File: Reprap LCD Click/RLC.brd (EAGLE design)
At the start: 100 x 80 mm, 10 parts, among them IC1 PCF8574T, Q1 BC548B, SW1 EC12E_SW, X1 HD44780LCD-1602

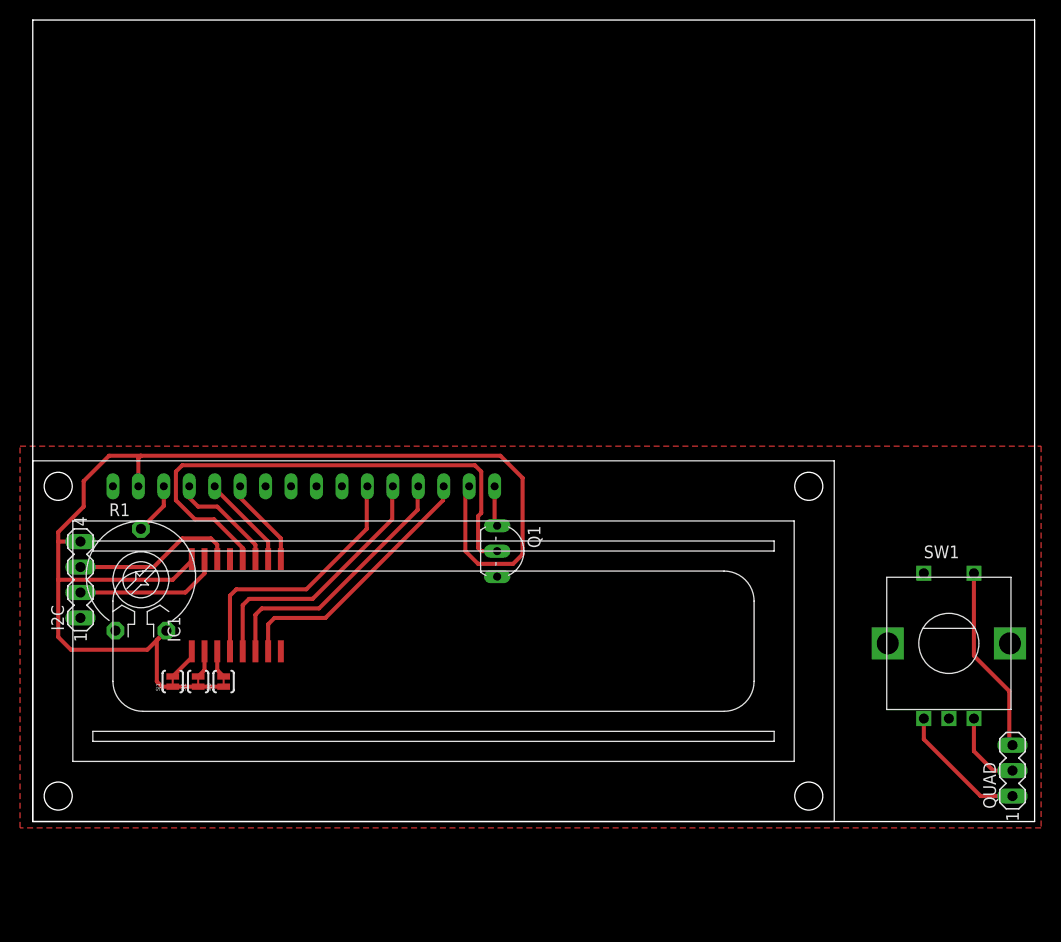
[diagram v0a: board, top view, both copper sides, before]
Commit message: r1v3, reprap LCD clicker, alvin board
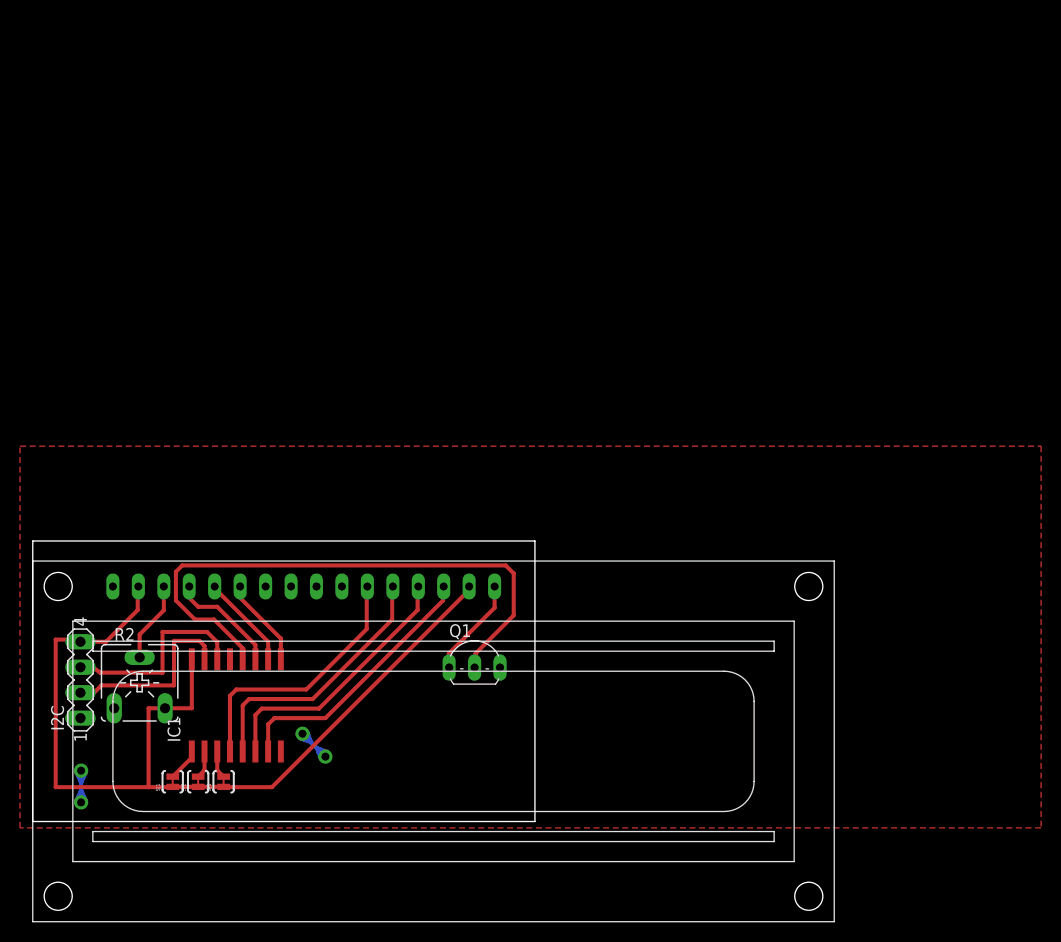
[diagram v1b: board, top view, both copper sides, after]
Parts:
- removed QUAD: (no value), con-lstb:MA03-1
- removed R1: (no value), rcl:PT-10
- removed SW1: EC12E_SW, switch-alps:ALPS_EC12E_SW
- added R2: (no value), pot:CA6V
- moved Q1 10.9 mm to (44.1, 16.6), turned to 0 degrees
- moved IC1 10.0 mm to (20.3, 11.6)
- moved SJ1 10.0 mm to (14.0, 3.97)
- moved SJ2 10.0 mm to (16.5, 3.97)
- moved SJ3 10.0 mm to (19.1, 3.97)
- moved X1 10.0 mm to (0.00, -10.0)
- moved I2C 10.00 mm to (4.76, 14.1)
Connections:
- removed net N$15: QUAD.3, SW1.E
- removed net N$16: QUAD.2, SW1.B
- removed net N$17: QUAD.1, SW1.A
- net +5V: now also R2.E; no longer R1.2
- net GND: now also R2.A; no longer R1.1, SW1.C, SW1.D
- net N$13: now also R2.S; no longer R1.3
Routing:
- net +5V: track 127.4 -> 93.6 mm
- net GND: track 0.00 -> 19.2 mm, vias 0 -> 4
- net N$15: track 18.8 -> 0.00 mm
- net N$17: track 13.3 -> 0.00 mm
- net N$16: track 7.91 -> 0.00 mm
- net N$12: track 4.04 -> 10.00 mm
- net N$11: track 53.4 -> 57.9 mm
- net SDA: track 14.6 -> 18.7 mm
- net SCL: track 16.5 -> 20.0 mm
- net N$13: track 5.20 -> 8.08 mm
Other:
- board size 100 x 80 mm -> 50.1 x 28 mm
